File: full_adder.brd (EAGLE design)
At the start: 100 x 120 mm, 91 parts, among them T101 TPH1R712MD, T102 TPH1R712MD, U1001 FDS6892A, U1002 FDS6892A, U1003 FDS6892A, U101 ATTINY45-20P, U201 CD4052BE, U202 CD4052BE, U203 CD4052BE, U401 KM28C65A-20, U501 74HC4051N,652, U601 NE555, U701 SN74LS74AN

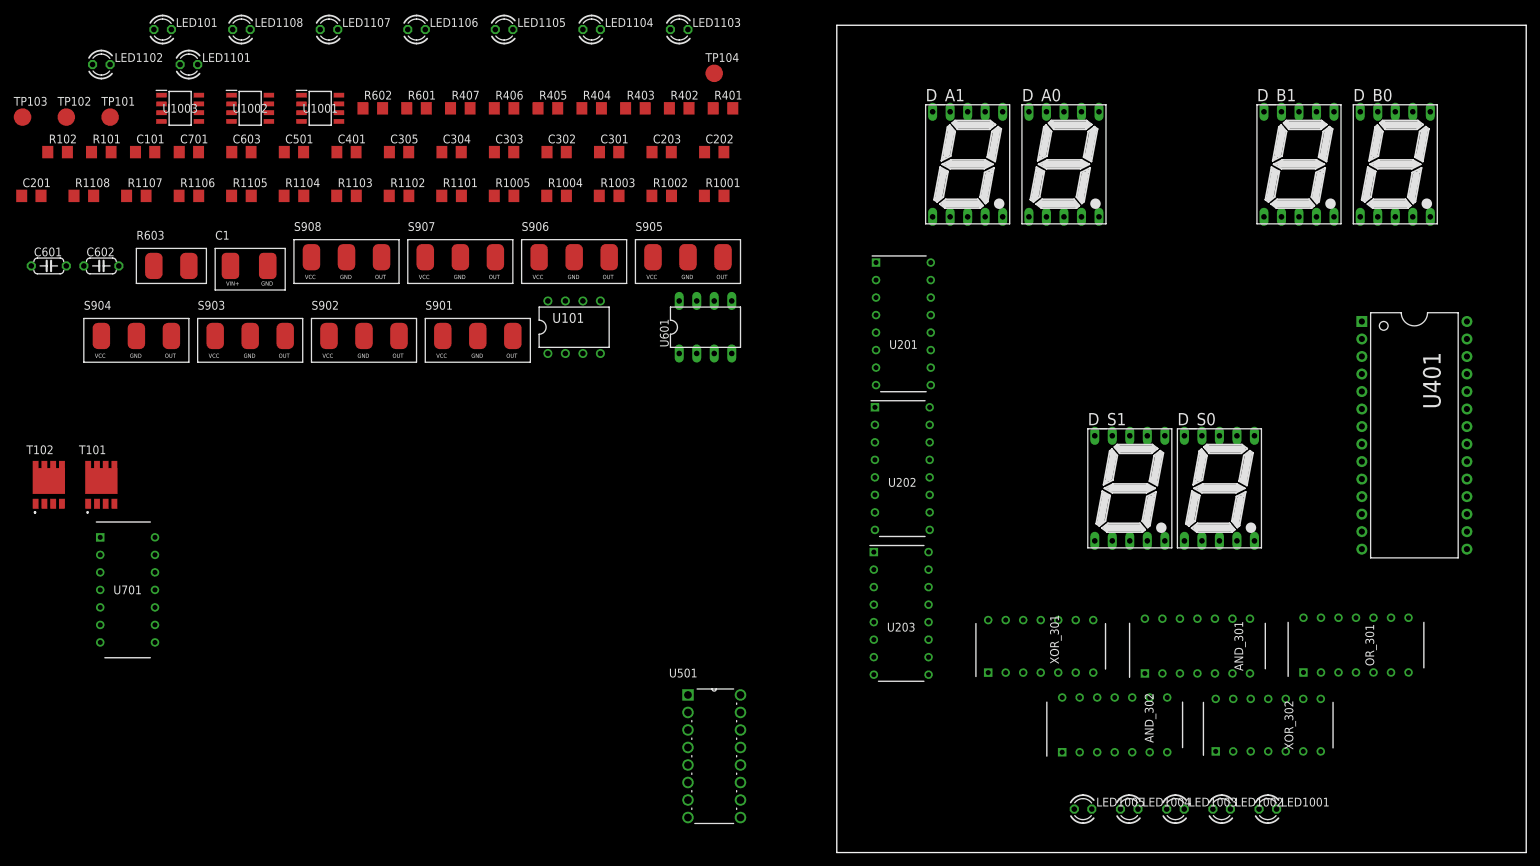
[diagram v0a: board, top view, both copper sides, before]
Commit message: basic layout complete
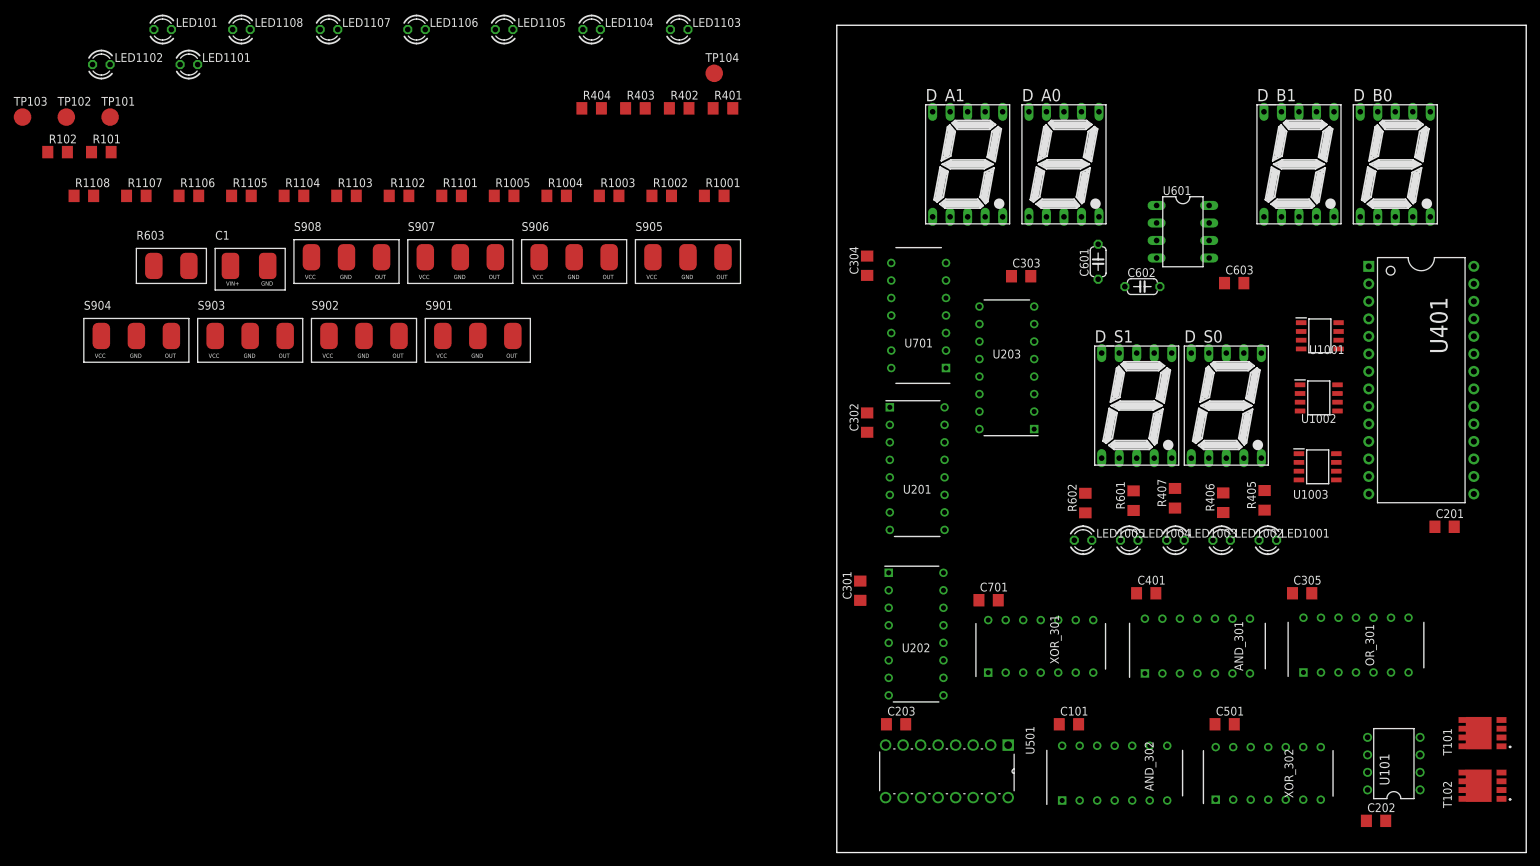
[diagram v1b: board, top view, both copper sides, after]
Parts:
- moved T102 212.5 mm to (93.7, 9.70), turned to 90 degrees
- moved C201 210.5 mm to (88.2, 47.2)
- moved T101 203.6 mm to (93.7, 17.3), turned to 90 degrees
- moved U1003 173.0 mm to (69.8, 56.0)
- moved U1002 160.6 mm to (69.9, 66.0)
- moved C501 158.5 mm to (56.3, 18.6)
- moved C101 157.6 mm to (33.7, 18.6)
- moved C601 152.2 mm to (37.9, 85.7), turned to 90 degrees
- moved C602 151.0 mm to (44.3, 82.1)
- moved U1001 148.7 mm to (70.1, 75.0)
- moved C305 145.8 mm to (67.5, 37.6)
- moved C603 145.2 mm to (57.6, 82.6)
- moved C202 136.5 mm to (78.2, 4.60)
- moved U101 134.7 mm to (80.8, 12.9), turned to 90 degrees
- moved C701 133.0 mm to (22.0, 36.6)
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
